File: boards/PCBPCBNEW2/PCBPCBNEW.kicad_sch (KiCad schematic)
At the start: 25 parts, among them J1 Screw_Terminal_01x02, J4 Screw_Terminal_01x06, U4 SIC431AED-T1-GE3

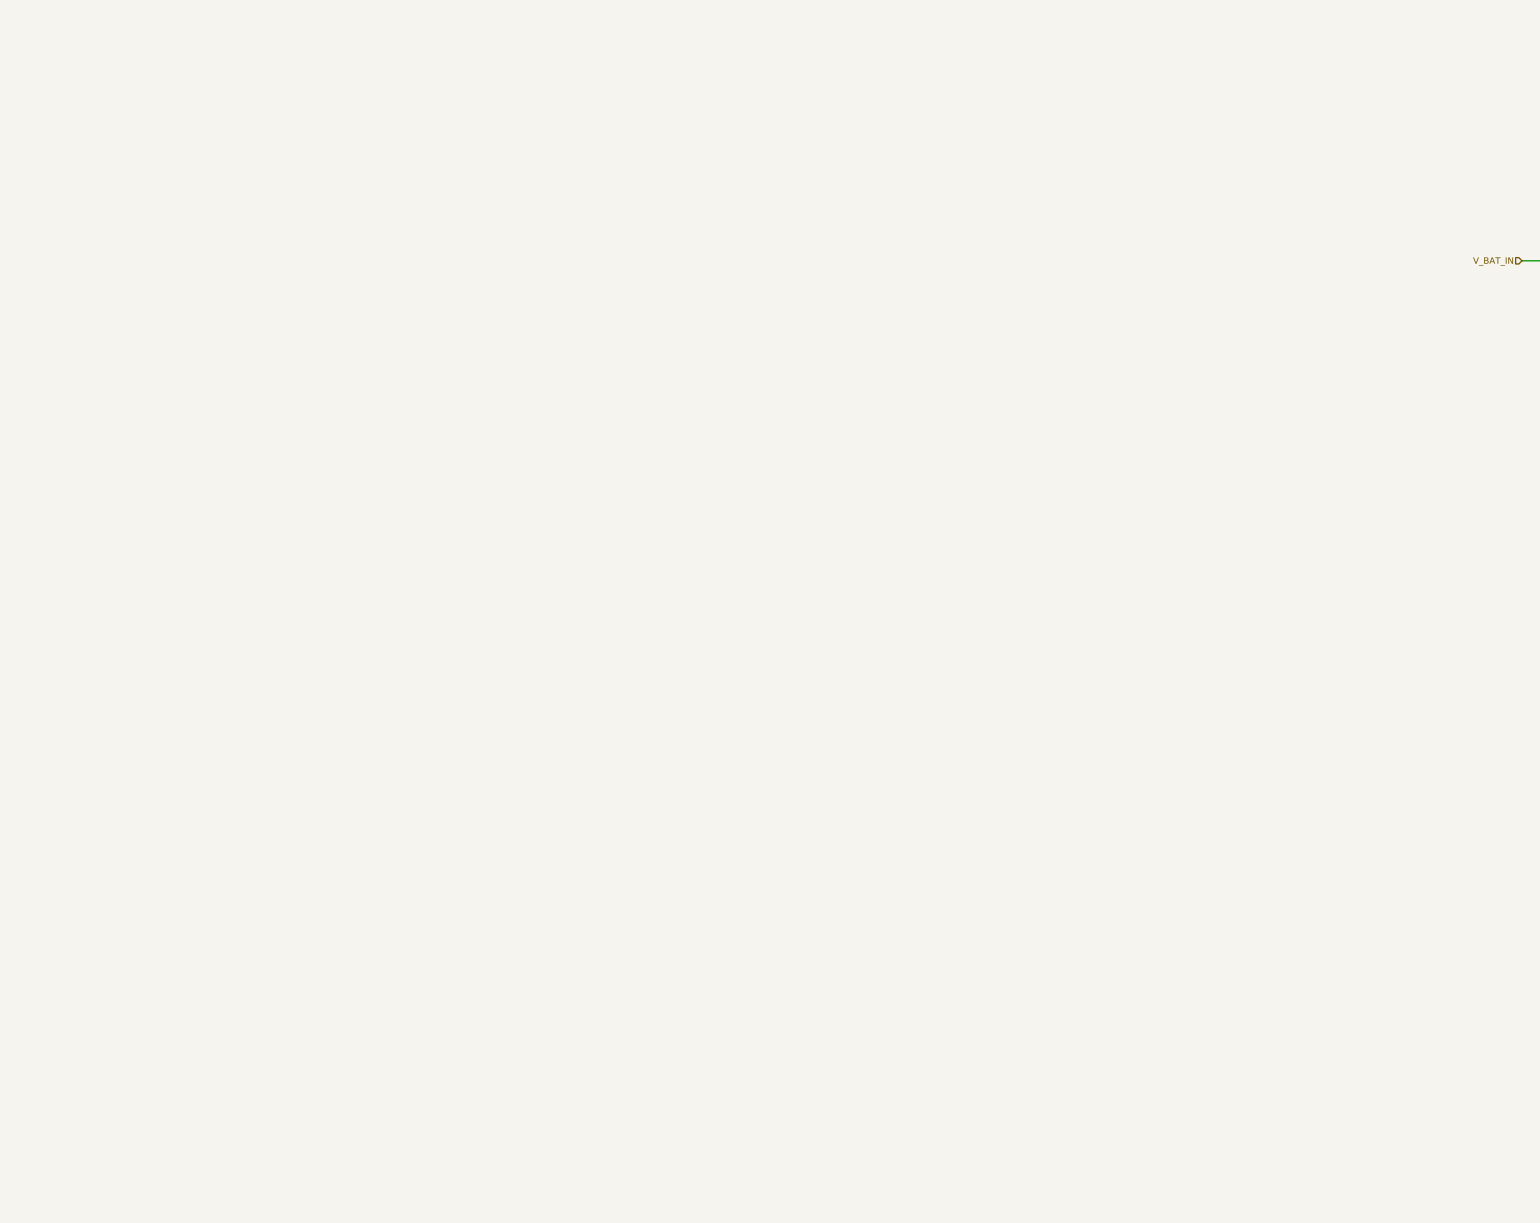
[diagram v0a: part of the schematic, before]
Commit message: Remade schematic and imported library
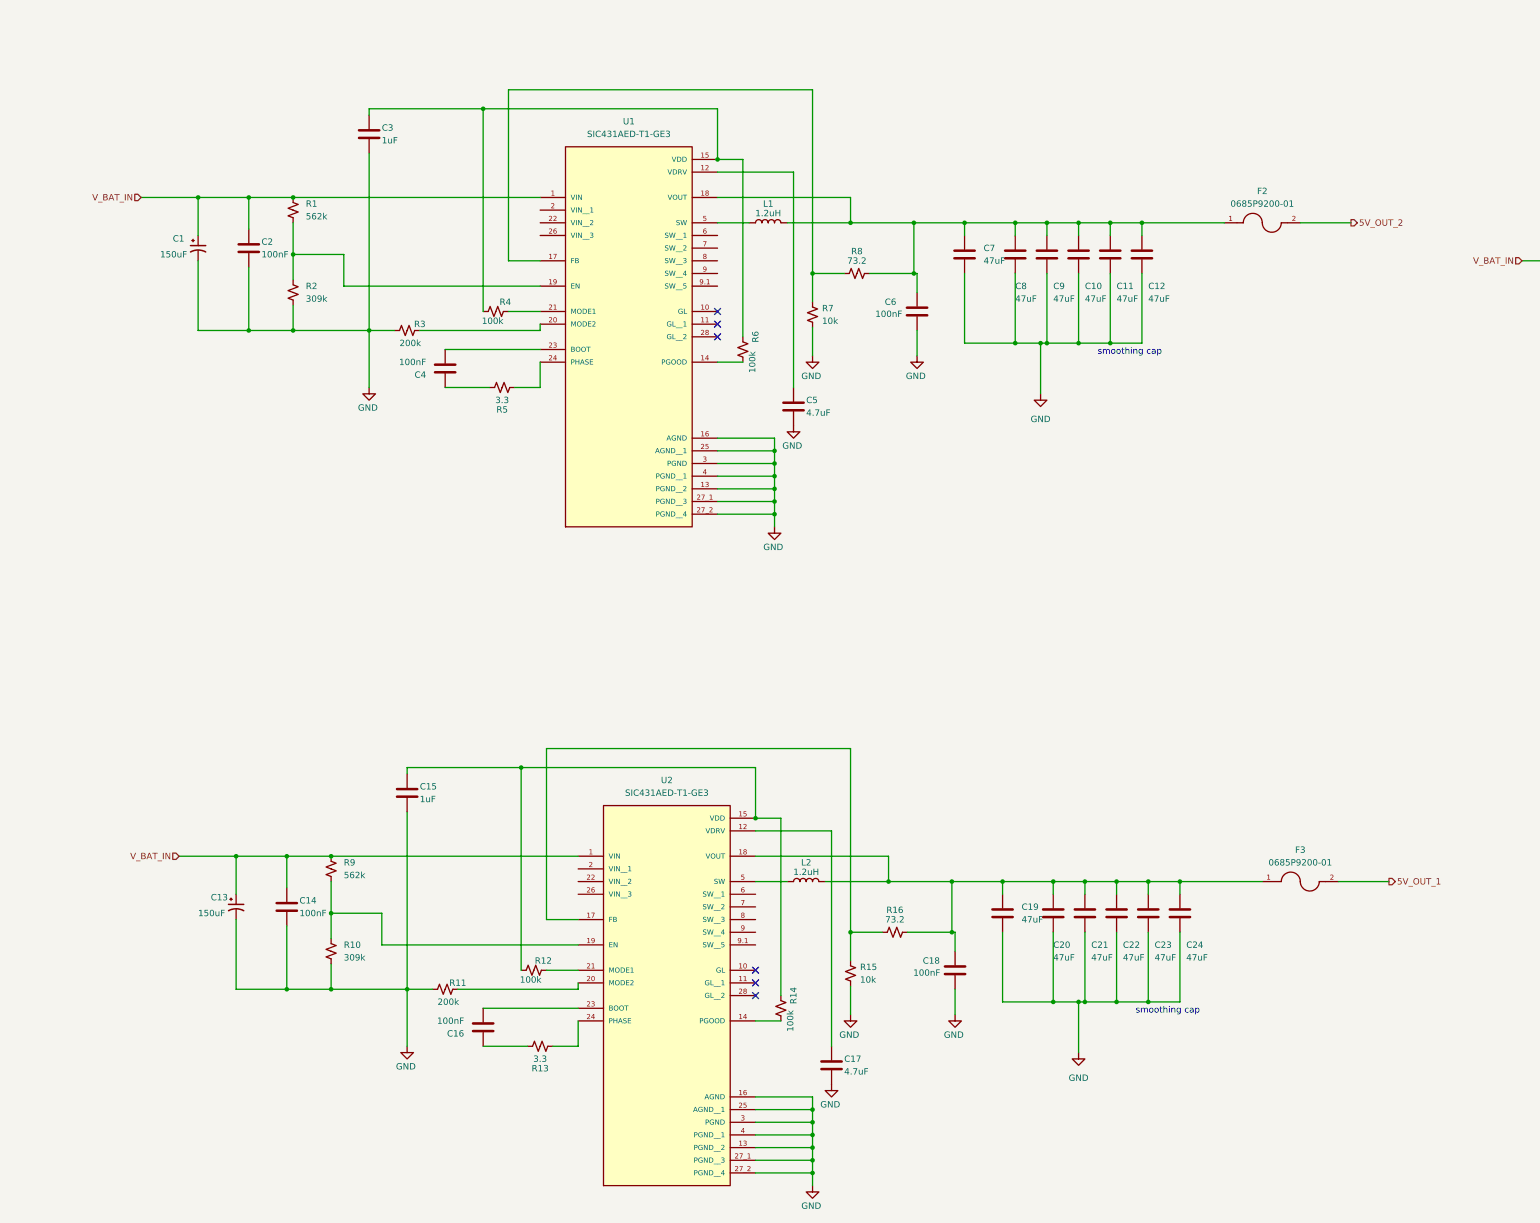
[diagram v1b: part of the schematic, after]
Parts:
- added C1, C13: 150uF, Capacitor_THT:CP_Radial_D12.5mm_P5.00mm, symbol Device:C_Polarized_Small_US
- added C10, C11, C12, C19, C20, C21, C22, C23, C24, C7, C8, C9: 47uF, Capacitor_SMD:C_0805_2012Metric, symbol Device:C
- added C14, C16, C18, C2, C4, C6: 100nF, Capacitor_SMD:C_0805_2012Metric, symbol Device:C
- added C15, C3: 1uF, Capacitor_SMD:C_0805_2012Metric, symbol Device:C
- added C17, C5: 4.7uF, Capacitor_SMD:C_0805_2012Metric, symbol Device:C
- added F2, F3: 0685P9200-01, 0685P9200_01:FUSC3215X83N, symbol 0685P9200-01:0685P9200-01
- added L1, L2: 1.2uH, Inductor_SMD:L_Vishay_IHLP-5050, symbol Device:L
- added R1, R9: 562k, Resistor_SMD:R_0805_2012Metric, symbol Device:R_Small_US
- added R10, R2: 309k, Resistor_SMD:R_0805_2012Metric, symbol Device:R_Small_US
- added R11, R3: 200k, Resistor_SMD:R_0805_2012Metric, symbol Device:R_Small_US
- added R12, R14, R4, R6: 100k, Resistor_SMD:R_0805_2012Metric, symbol Device:R_Small_US
- added R13, R5: 3.3, Resistor_SMD:R_0805_2012Metric, symbol Device:R_Small_US
- added R15, R7: 10k, Resistor_SMD:R_0805_2012Metric, symbol Device:R_Small_US
- added R16, R8: 73.2, Resistor_SMD:R_0805_2012Metric, symbol Device:R_Small_US
- added U1, U2: SIC431AED-T1-GE3, SIC431AED_T1_GE3:REGULATOR_SIC431AED-T1-GE3, symbol SIC431AED-T1-GE3:SIC431AED-T1-GE3
- J1: footprint power_board_support:TE_1986660-2 -> REAAAL:TE_1986660-2a
- J4: footprint power_board_support:691137710006 -> REAAAL:TEST2
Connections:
- net 5V_OUT_1: now also F3.2
- net 5V_OUT_2: now also F2.2
- net GND: now also C1.2, C10.2, C11.2, C12.2, C13.2, C14.2, C15.2, C17.2, C18.2, C19.2, C2.2, C20.2, C21.2, C22.2, C23.2, C24.2, C3.2, C5.2, C6.2, C7.2, C8.2, C9.2, R10.2, R11.1, R15.2, R2.2, R3.1, R7.2, U1.13 (PGND__2), U1.16 (AGND), U1.25 (AGND__1), U1.27_1 (PGND__3), U1.27_2 (PGND__4), U1.3 (PGND), U1.4 (PGND__1), U2.13 (PGND__2), U2.16 (AGND), U2.25 (AGND__1), U2.27_1 (PGND__3), U2.27_2 (PGND__4), U2.3 (PGND), U2.4 (PGND__1)
- net V_BAT_IN: now also C1.1, C13.1, C14.1, C2.1, R1.1, R9.1, U1.1 (VIN), U2.1 (VIN)
- new net: C18.1, C19.1, C20.1, C21.1, C22.1, C23.1, C24.1, F3.1, L2.2, R16.2, U2.18 (VOUT)
- new net: C3.1, R4.1, R6.1, U1.15 (VDD)
- new net: R6.2, U1.14 (PGOOD)
- new net: C10.1, C11.1, C12.1, C6.1, C7.1, C8.1, C9.1, F2.1, L1.2, R8.2, U1.18 (VOUT)
- new net: L2.1, U2.5 (SW)
- new net: R3.2, U1.20 (MODE2)
- new net: R15.1, R16.1, U2.17 (FB)
- new net: R13.1, U2.24 (PHASE)
- new net: C16.1, R13.2
- new net: C17.1, U2.12 (VDRV)
- new net: R14.2, U2.14 (PGOOD)
- new net: C15.1, R12.1, R14.1, U2.15 (VDD)
- new net: R10.1, R9.2, U2.19 (EN)
- new net: R11.2, U2.20 (MODE2)
- new net: R12.2, U2.21 (MODE1)
- new net: C16.2, U2.23 (BOOT)
- new net: R1.2, R2.1, U1.19 (EN)
- new net: C4.1, R5.2
- new net: C4.2, U1.23 (BOOT)
- new net: R4.2, U1.21 (MODE1)
- new net: R5.1, U1.24 (PHASE)
- new net: R7.1, R8.1, U1.17 (FB)
- new net: L1.1, U1.5 (SW)
- new net: C5.1, U1.12 (VDRV)
- no-connect marks 3 -> 9
